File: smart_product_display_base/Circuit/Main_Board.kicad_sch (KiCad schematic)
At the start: 43 parts, among them Q1 BD681, Q2 BD681, Q3 BD681, Q4 BD681, Q5 BD681, Q6 BD681, U1 PC817, U2 PC817, U3 PC817, U4 PC817, U5 PC817, U6 PC817

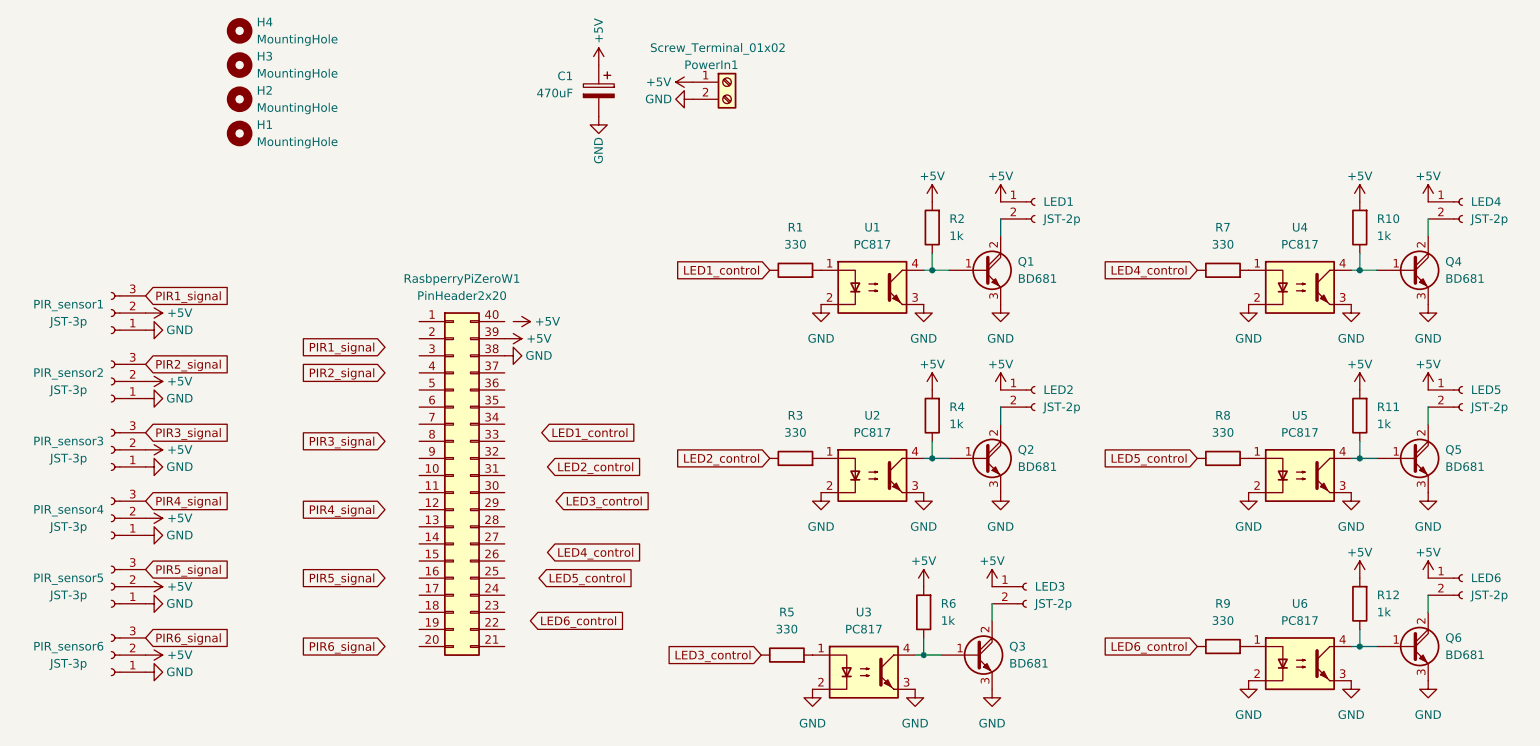
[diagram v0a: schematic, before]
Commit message: finished PCB layout
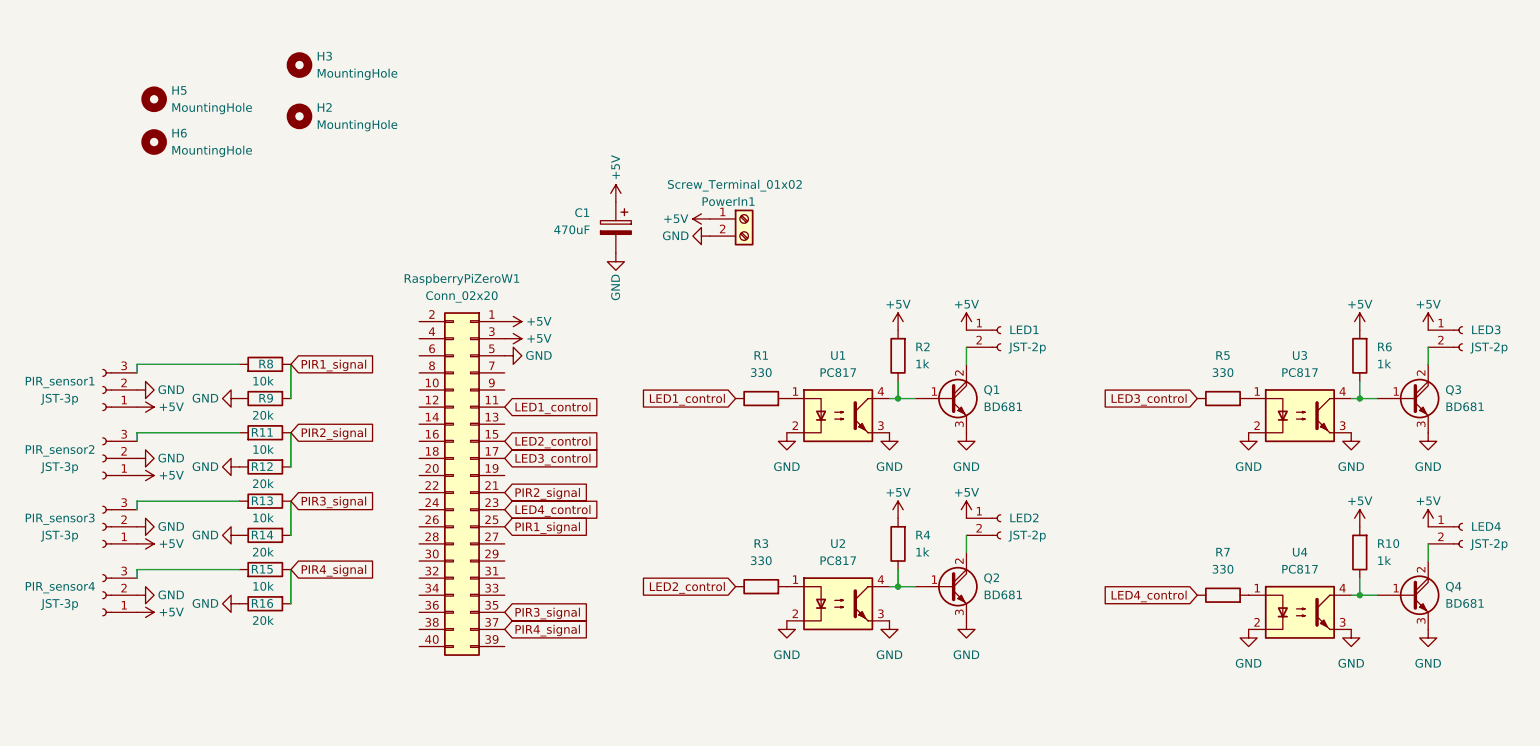
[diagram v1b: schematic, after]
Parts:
- removed H1, H4: MountingHole, MountingHole:MountingHole_5.5mm_Pad_TopBottom, symbol Mechanical:MountingHole
- removed LED5, LED6: JST-2p, Connector_JST:JST_EH_B2B-EH-A_1x02_P2.50mm_Vertical, symbol Connector:Conn_01x02_Socket
- removed PIR_sensor5, PIR_sensor6: JST-3p, Connector_JST:JST_EH_B3B-EH-A_1x03_P2.50mm_Vertical, symbol Connector:Conn_01x03_Socket
- removed Q5, Q6: BD681, Package_TO_SOT_THT:TO-126-3_Vertical, symbol Device:Q_NPN_Darlington_BCE
- removed RasbperryPiZeroW1: PinHeader2x20, Connector_PinSocket_2.54mm:PinSocket_2x20_P2.54mm_Vertical, symbol Connector_Generic:Conn_02x20_Counter_Clockwise
- removed U5, U6: PC817, Package_DIP:DIP-4_W7.62mm, symbol Isolator:PC817
- added H5, H6: MountingHole, MountingHole:MountingHole_2.5mm_Pad_TopOnly, symbol Mechanical:MountingHole
- added R13, R15: 10k, Resistor_THT:R_Axial_DIN0207_L6.3mm_D2.5mm_P7.62mm_Horizontal, symbol Device:R
- added R14, R16: 20k, Resistor_THT:R_Axial_DIN0207_L6.3mm_D2.5mm_P7.62mm_Horizontal, symbol Device:R
- added RaspberryPiZeroW1: Conn_02x20, Connector_PinSocket_2.54mm:PinSocket_2x20_P2.54mm_Vertical, symbol Connector_Generic:Conn_02x20_Odd_Even
- H2, H3: footprint MountingHole:MountingHole_5.5mm_Pad_TopBottom -> MountingHole:MountingHole_4mm_Pad_TopOnly
- R11: value 1k -> 10k
- R12: value 1k -> 20k
- R8: value 330 -> 10k
- R9: value 330 -> 20k
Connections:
- net LED5_control is gone; now on net PIR1_signal: R8.1
- net LED6_control is gone; now on net GND: R9.1
- net +5V: now also PIR_sensor1.1 (Pin_1), PIR_sensor2.1 (Pin_1), PIR_sensor3.1 (Pin_1), PIR_sensor4.1 (Pin_1), RaspberryPiZeroW1.1 (Pin_1), RaspberryPiZeroW1.3 (Pin_3); no longer PIR_sensor1.2 (Pin_2), PIR_sensor2.2 (Pin_2), PIR_sensor3.2 (Pin_2), PIR_sensor4.2 (Pin_2), R11.2, R12.2
- net GND: now also PIR_sensor1.2 (Pin_2), PIR_sensor2.2 (Pin_2), PIR_sensor3.2 (Pin_2), PIR_sensor4.2 (Pin_2), R12.1, R14.1, R16.1, RaspberryPiZeroW1.5 (Pin_5); no longer PIR_sensor1.1 (Pin_1), PIR_sensor2.1 (Pin_1), PIR_sensor3.1 (Pin_1), PIR_sensor4.1 (Pin_1)
- net LED1_control: now also RaspberryPiZeroW1.11 (Pin_11)
- net LED2_control: now also RaspberryPiZeroW1.15 (Pin_15)
- net LED3_control: now also RaspberryPiZeroW1.17 (Pin_17)
- net LED4_control: now also RaspberryPiZeroW1.23 (Pin_23)
- net PIR1_signal: now also R9.2, RaspberryPiZeroW1.25 (Pin_25); no longer PIR_sensor1.3 (Pin_3)
- net PIR2_signal: now also R11.1, R12.2, RaspberryPiZeroW1.21 (Pin_21); no longer PIR_sensor2.3 (Pin_3)
- net PIR3_signal: now also R13.1, R14.2, RaspberryPiZeroW1.35 (Pin_35); no longer PIR_sensor3.3 (Pin_3)
- net PIR4_signal: now also R15.1, R16.2, RaspberryPiZeroW1.37 (Pin_37); no longer PIR_sensor4.3 (Pin_3)
- net at R8.2: now also PIR_sensor1.3 (Pin_3)
- new net: PIR_sensor4.3 (Pin_3), R15.2
- new net: PIR_sensor2.3 (Pin_3), R11.2
- new net: PIR_sensor3.3 (Pin_3), R13.2
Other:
- moved on the sheet: C1, LED1, LED2, LED3, LED4, PIR_sensor1, PIR_sensor2, PIR_sensor3, PIR_sensor4, PowerIn1, Q1, Q2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
